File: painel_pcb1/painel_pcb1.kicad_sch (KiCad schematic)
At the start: 59 parts, among them J1 Conn_02x16_Counter_Clockwise, J2 Conn_02x02_Counter_Clockwise, J3 Conn_02x06_Counter_Clockwise, J4 Conn_02x08_Counter_Clockwise, J5 Conn_02x03_Counter_Clockwise, J6 Conn_02x08_Counter_Clockwise, J7 Conn_02x18_Counter_Clockwise, U1 MAX7219, U2 MAX7219, U3 74LS595, U4 74LS595, U5 Pico

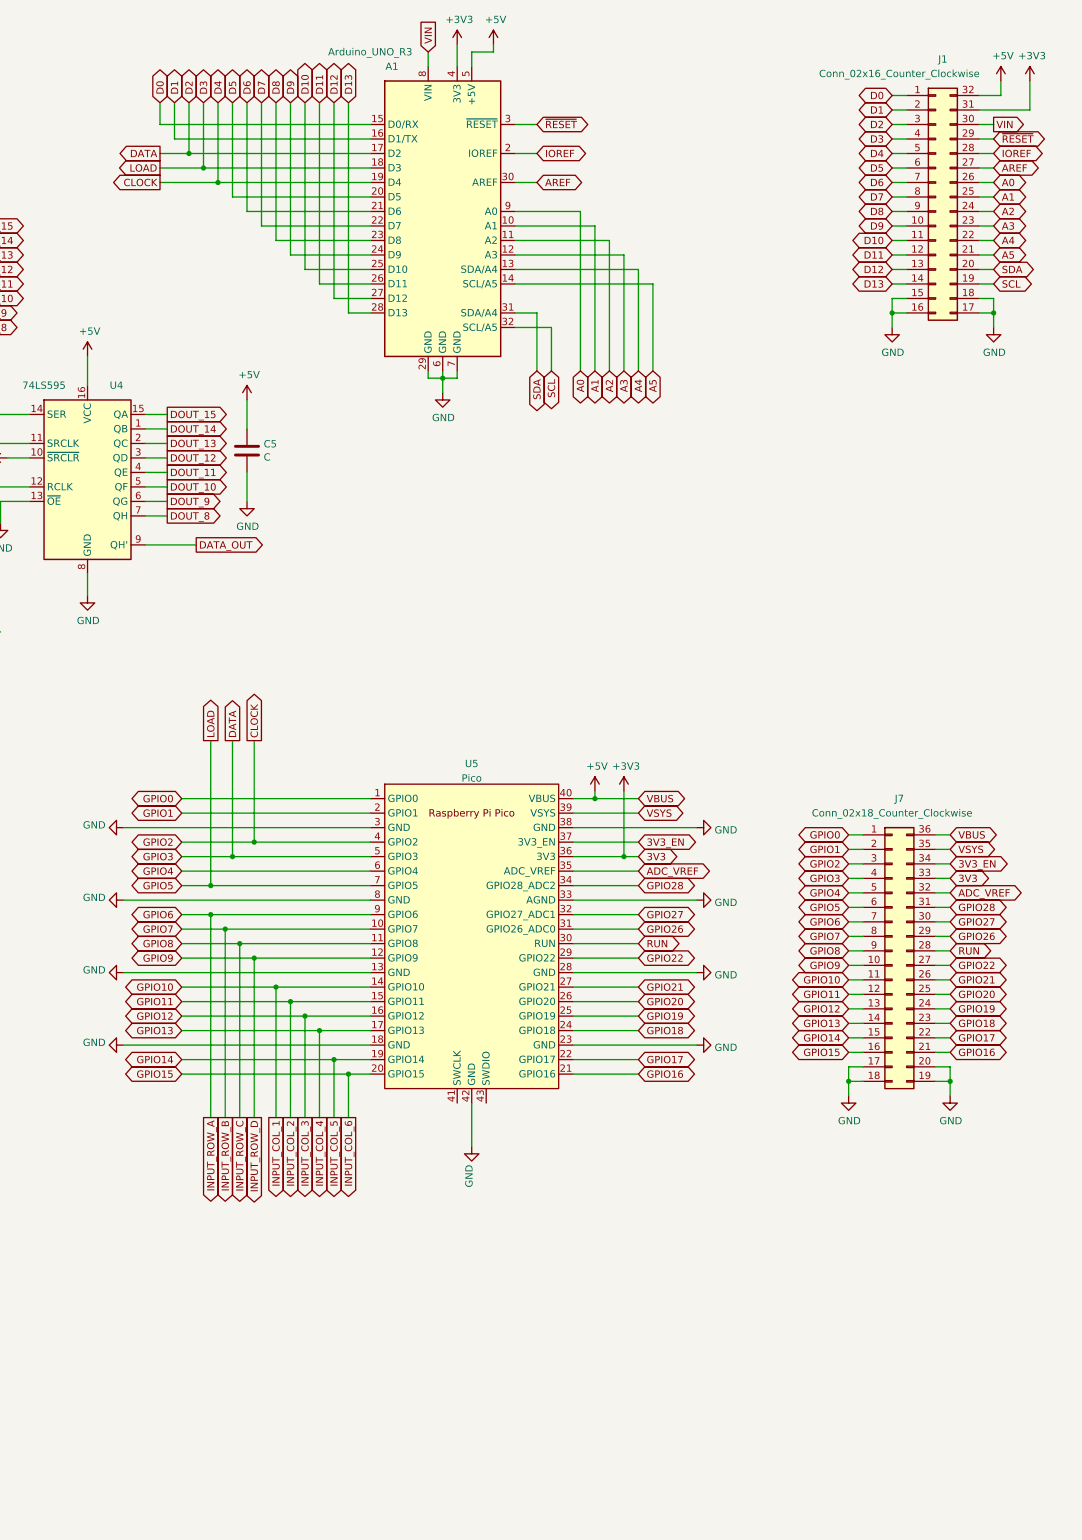
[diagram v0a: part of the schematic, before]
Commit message: autorouting
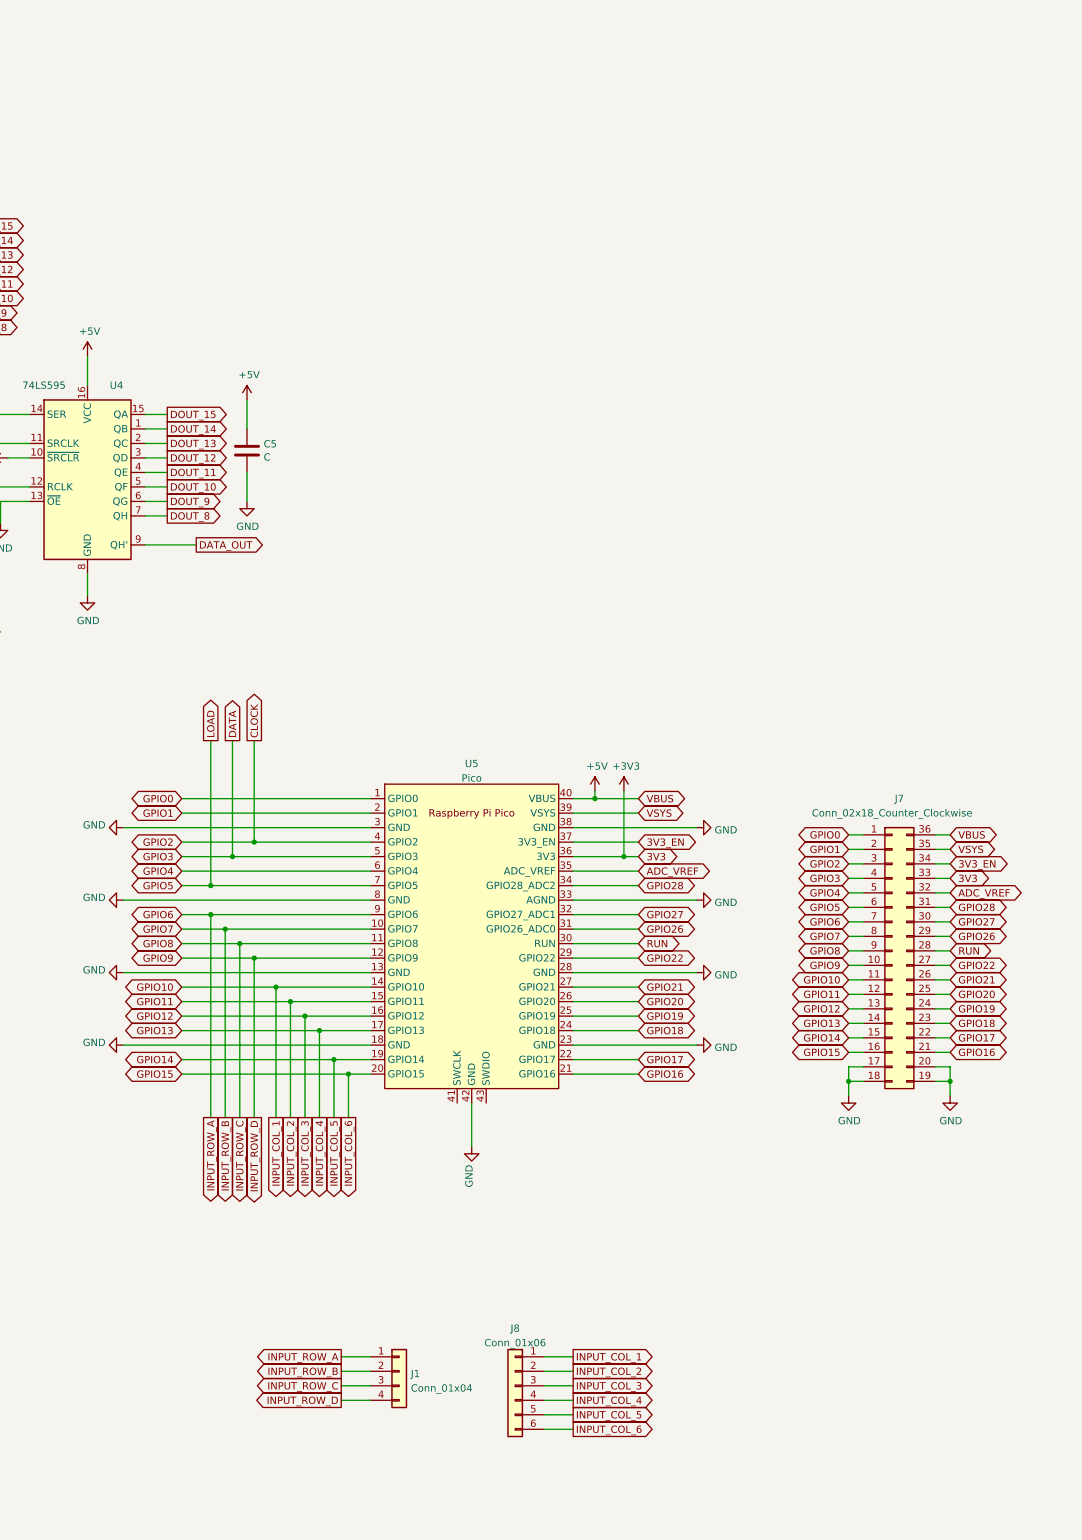
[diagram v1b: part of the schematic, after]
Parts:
- removed A1: Arduino_UNO_R3, Module:Arduino_UNO_R3, symbol MCU_Module:Arduino_UNO_R3
- removed J1: Conn_02x16_Counter_Clockwise, Connector_PinHeader_2.54mm:PinHeader_2x16_P2.54mm_Vertical, symbol Connector_Generic:Conn_02x16_Counter_Clockwise
- added J1: Conn_01x04, Connector_PinHeader_2.54mm:PinHeader_1x04_P2.54mm_Vertical, symbol Connector_Generic:Conn_01x04
- added J8: Conn_01x06, Connector_PinHeader_2.54mm:PinHeader_1x06_P2.54mm_Vertical, symbol Connector_Generic:Conn_01x06
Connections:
- net GPIO10: now also J8.1 (Pin_1)
- net GPIO11: now also J8.2 (Pin_2)
- net GPIO12: now also J8.3 (Pin_3)
- net GPIO13: now also J8.4 (Pin_4)
- net GPIO14: now also J8.5 (Pin_5)
- net GPIO15: now also J8.6 (Pin_6)
- net GPIO6: now also J1.1 (Pin_1)
- net GPIO7: now also J1.2 (Pin_2)
- net GPIO8: now also J1.3 (Pin_3)
- net GPIO9: now also J1.4 (Pin_4)
- net D2 renamed DATA
- net D3 renamed GPIO5
